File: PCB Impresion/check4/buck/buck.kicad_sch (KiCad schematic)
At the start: 8 parts, among them J1 OUT, J2 OUT, J3 OUT, Q1 IRF3205, Q2 IRF3205

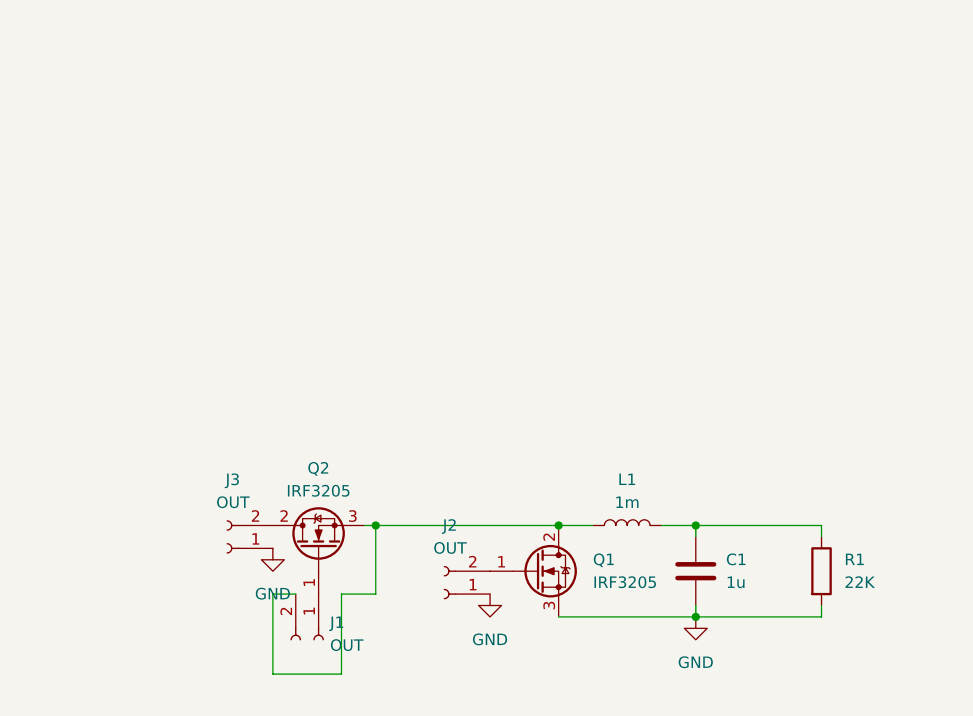
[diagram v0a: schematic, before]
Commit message: pcb buck
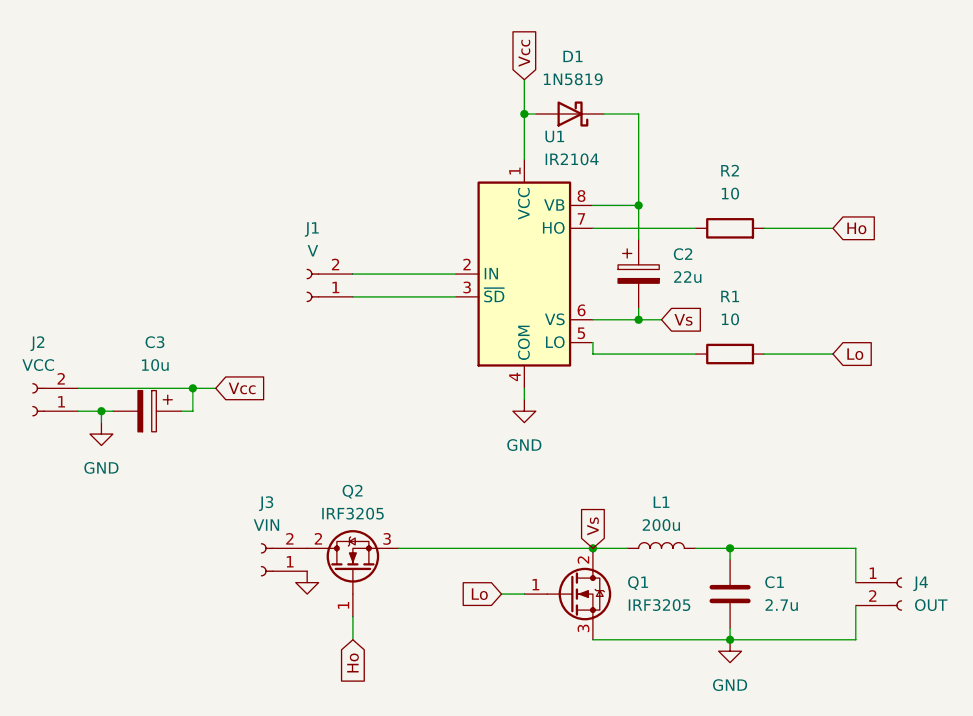
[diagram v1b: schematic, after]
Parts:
- added C2: 22u, Capacitor_THT:CP_Radial_D6.3mm_P2.50mm, symbol Device:C_Polarized
- added C3: 10u, Capacitor_THT:CP_Radial_D6.3mm_P2.50mm, symbol Device:C_Polarized
- added D1: 1N5819, Diode_THT:D_DO-41_SOD81_P10.16mm_Horizontal, symbol Diode:1N5819
- added J4: OUT, TerminalBlock_Phoenix:TerminalBlock_Phoenix_MKDS-3-2-5.08_1x02_P5.08mm_Horizontal, symbol Connector:Conn_01x02_Socket
- added R2: 10, Resistor_THT:R_Axial_DIN0204_L3.6mm_D1.6mm_P7.62mm_Horizontal, symbol Device:R
- added U1: IR2104, Package_DIP:CERDIP-8_W7.62mm_SideBrazed_LongPads_Socket, symbol Driver_FET:IR2104
- C1: value 1u -> 2.7u
- J1: value OUT -> V
- J2: value OUT -> VCC
- J3: value OUT -> VIN
- L1: value 1m -> 200u; footprint Inductor_THT:L_Axial_L6.6mm_D2.7mm_P10.16mm_Horizontal_Vishay_IM-2 -> Inductor_THT:L_Toroid_Vertical_L16.5mm_W11.4mm_P7.62mm_Pulse_KM-2
- R1: value 22K -> 10
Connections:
- net GND: now also C3.2, J4.2 (Pin_2), U1.4 (COM); no longer R1.2
- net Lo: now reaches Q1.1 (G)
- net Lo: now also R1.2; no longer J2.2 (Pin_2)
- net at J1.1 (Pin_1): now also U1.3 (~{SD}); no longer Q2.1 (G)
- net Vs: now reaches L1.1, Q1.2 (D), Q2.3 (S)
- net Vs: now also C2.2, U1.6 (VS); no longer J1.2 (Pin_2)
- net at C1.2, L1.2: now also J4.1 (Pin_1); no longer R1.1
- new net: C2.1, D1.1 (K), U1.8 (VB)
- new net: J1.2 (Pin_2), U1.2 (IN)
- new net: R1.1, U1.5 (LO)
- new net: R2.1, U1.7 (HO)
- new net Ho: Q2.1 (G), R2.2
- new net Vcc: C3.1, D1.2 (A), J2.2 (Pin_2), U1.1 (VCC)
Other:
- moved on the sheet: C1, J3, L1, Q1, Q2
